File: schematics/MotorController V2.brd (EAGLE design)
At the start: 120.6 x 100 mm, 51 parts, among them IC1 7805, Q1 BC307

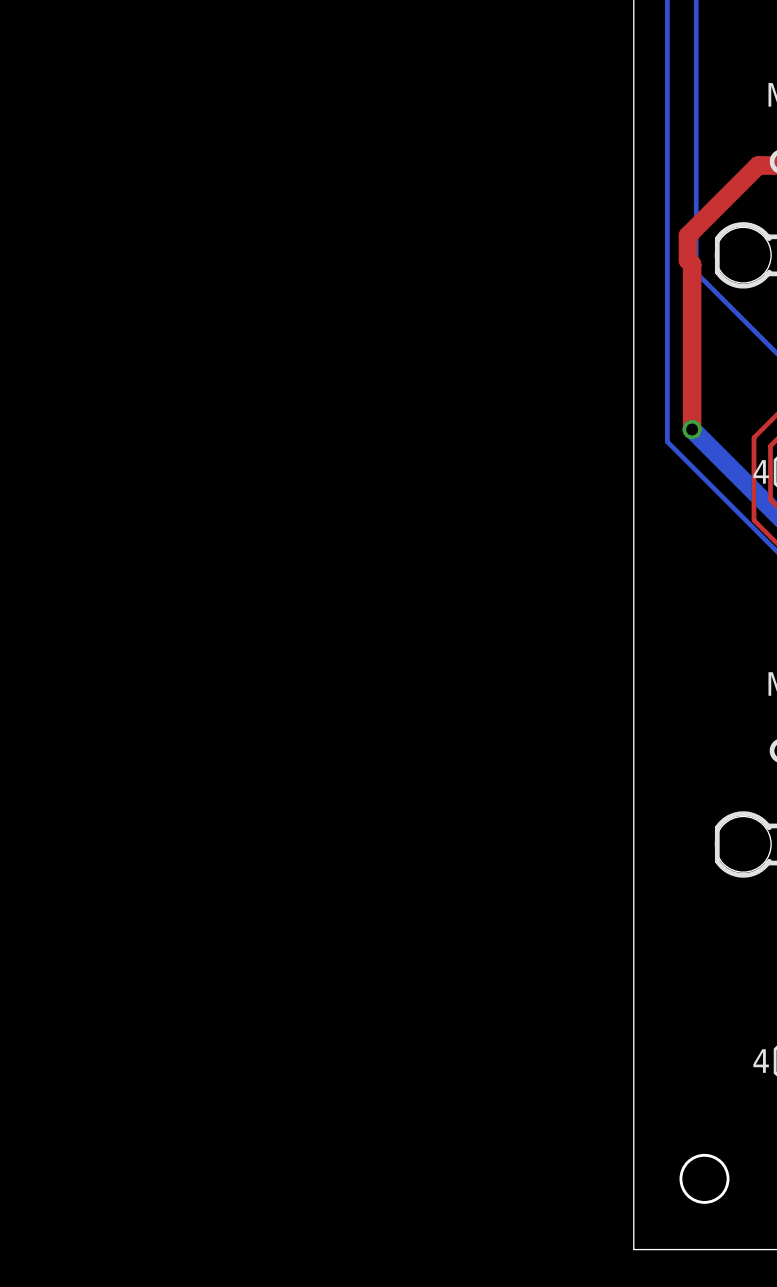
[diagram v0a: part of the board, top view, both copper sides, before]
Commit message: no message
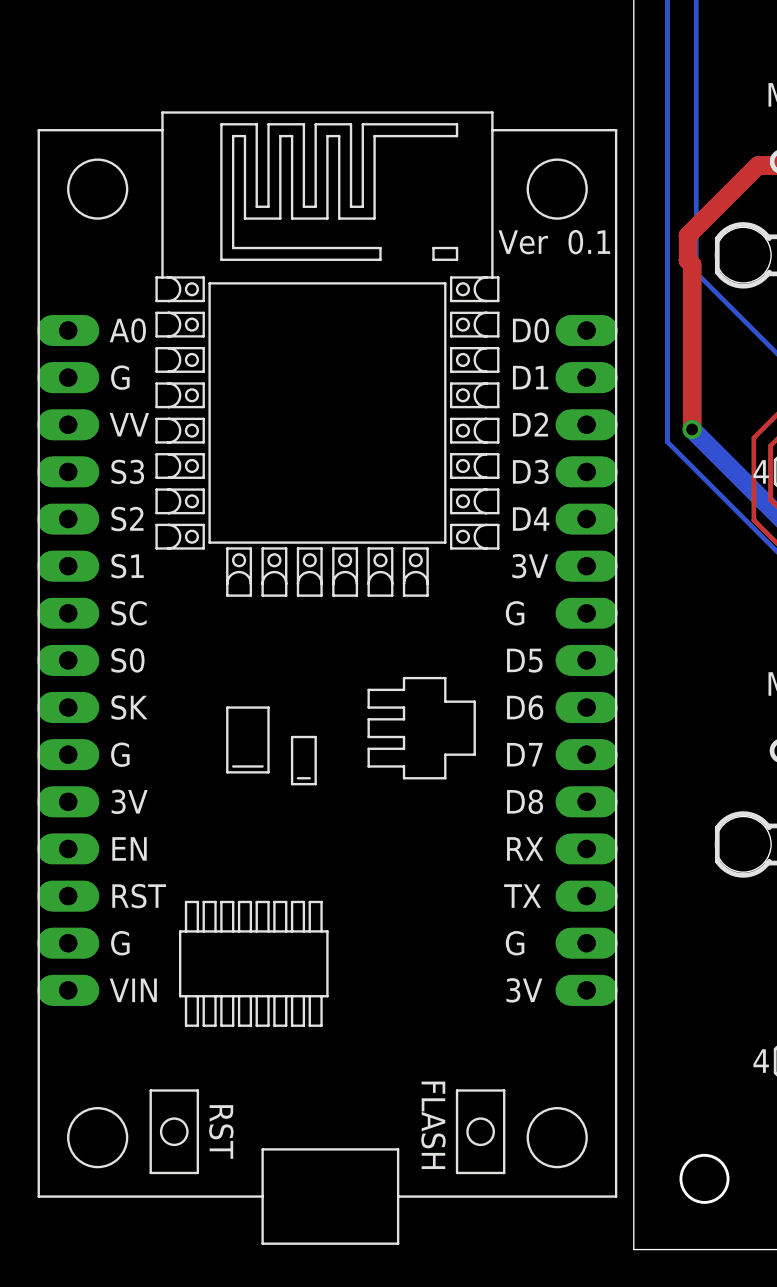
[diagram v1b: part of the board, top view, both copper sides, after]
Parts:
- added U$3: NODEMCU, nodemcu:NODEMCU
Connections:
- new net 3V: U$3.11, U$3.16, U$3.25
- net GND: now also U$3.10, U$3.14, U$3.17, U$3.2, U$3.24
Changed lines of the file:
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@@
 <element name="D12" library="diode" library_urn="urn:adsk.eagle:library:210" package="DO41Z10" package3d_urn="urn:adsk.eagle:package:43341/1" value="5.6V" x="-46.355" y="6.35" rot="R180"/>
 <element name="D13" library="diode" library_urn="urn:adsk.eagle:library:210" package="DO41Z10" package3d_urn="urn:adsk.eagle:package:43341/1" value="5.6V" x="-46.355" y="3.81" rot="R180"/>
+<element name="U$3" library="nodemcu" package="NODEMCU" value="NODEMCU" x="-91.44" y="17.78"/>
 </elements>
 <signals>
@@
 <wire x1="-15.113" y1="77.56525" x2="-15.24" y2="77.47" width="0.254" layer="1"/>
 <wire x1="38.00475" y1="71.12" x2="38.1" y2="71.12" width="0.254" layer="1"/>
+<contactref element="U$3" pad="2"/>
+<contactref element="U$3" pad="10"/>
+<contactref element="U$3" pad="14"/>
+<contactref element="U$3" pad="17"/>
+<contactref element="U$3" pad="24"/>
+<wire x1="-105.41" y1="12.7" x2="-105.41" y2="2.54" width="0" layer="19" extent="1-1"/>
+<wire x1="-105.41" y1="33.02" x2="-105.41" y2="12.7" width="0" layer="19" extent="1-1"/>
+<wire x1="-77.47" y1="2.54" x2="-105.41" y2="2.54" width="0" layer="19" extent="1-1"/>
+<wire x1="-66.00825" y1="-3.33375" x2="-77.47" y2="2.54" width="0" layer="19" extent="16-16"/>
+<wire x1="-77.47" y1="20.32" x2="-66.2305" y2="28.0035" width="0" layer="19" extent="16-16"/>
 </signal>
 <signal name="N$4">
@@
 <wire x1="-29.337" y1="42.00525" x2="-29.21" y2="41.91" width="0.254" layer="1"/>
 </signal>
+<signal name="3V">
+<contactref element="U$3" pad="11"/>
+<contactref element="U$3" pad="16"/>
+<contactref element="U$3" pad="25"/>
+<wire x1="-77.47" y1="0" x2="-105.41" y2="10.16" width="0" layer="19" extent="1-1"/>
+<wire x1="-77.47" y1="22.86" x2="-77.47" y2="0" width="0" layer="19" extent="1-1"/>
+</signal>
 </signals>
